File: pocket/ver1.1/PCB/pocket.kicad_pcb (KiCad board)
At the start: 2 copper layers, 225.4 x 60.3 mm, 60 parts, among them SW1 MX_SW_HS, SW10 MX_SW_HS, SW11 MX_SW_HS, SW12 MX_SW_HS, SW13 MX_SW_HS, SW14 MX_SW_HS, SW15 MX_SW_HS, SW16 MX_SW_HS, SW17 MX_SW_HS, SW18 MX_SW_HS, SW19 MX_SW_HS, SW2 MX_SW_HS, SW20 MX_SW_HS, SW21 MX_SW_HS, SW22 MX_SW_HS, SW23 MX_SW_HS, SW24 MX_SW_HS, SW25 MX_SW_HS, SW26 MX_SW_HS, SW27 MX_SW_HS, SW28 MX_SW_HS, SW29 MX_SW_HS, SW3 MX_SW_HS, SW4 MX_SW_HS, SW5 MX_SW_HS, SW6 MX_SW_HS, SW7 MX_SW_HS, SW8 MX_SW_HS, SW9 MX_SW_HS, U1 ProMicro

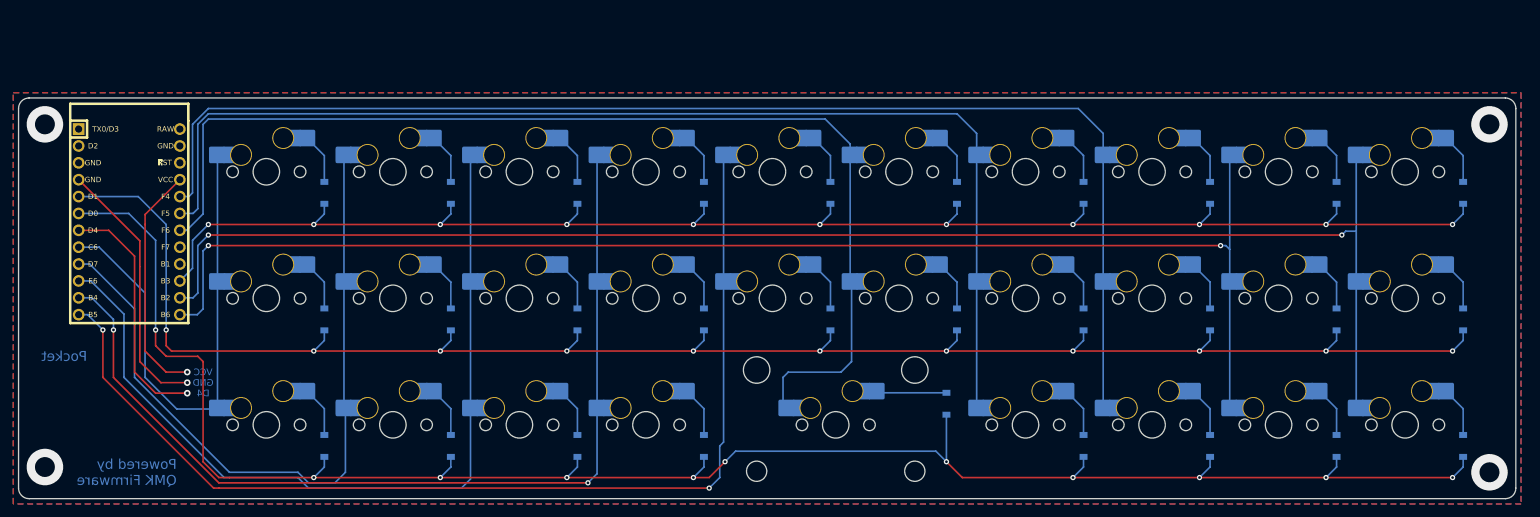
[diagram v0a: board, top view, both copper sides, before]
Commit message: Add files via upload
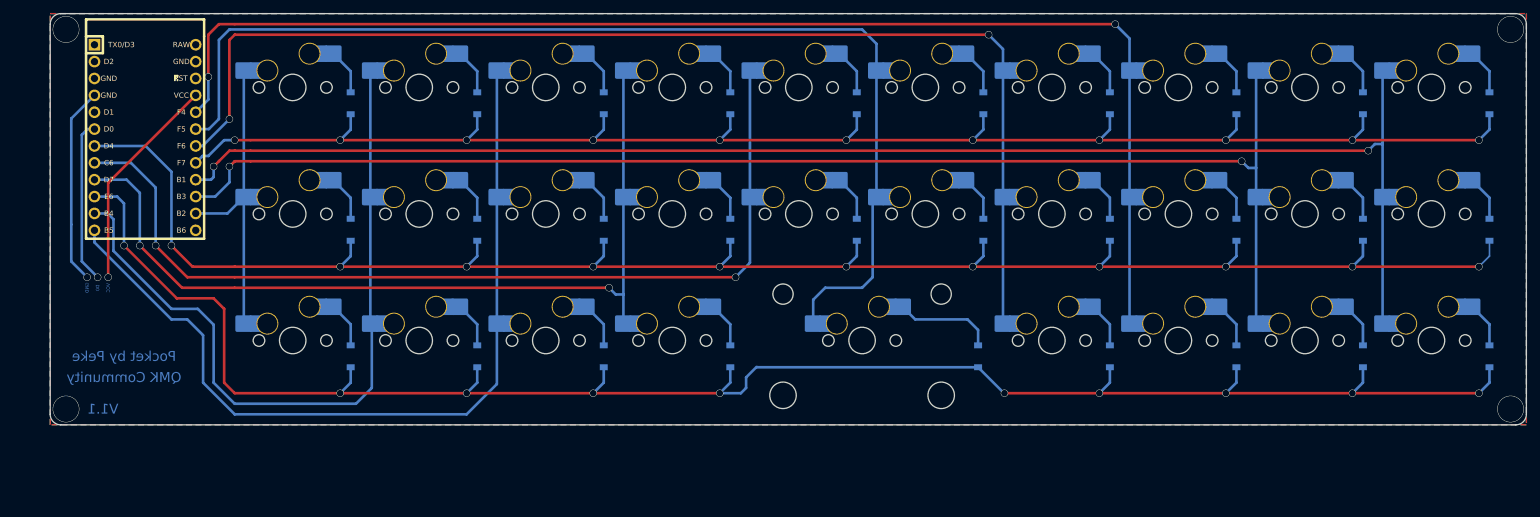
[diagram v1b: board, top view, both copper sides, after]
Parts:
- moved D1 14.1 mm to (261.1, 74.6)
- moved D10 14.1 mm to (89.7, 74.6)
- moved D11 14.1 mm to (261.1, 93.7)
- moved D12 14.1 mm to (242.1, 93.7)
- moved D13 14.1 mm to (223.0, 93.7)
- moved D14 14.1 mm to (204.0, 93.7)
- moved D15 14.1 mm to (184.9, 93.7)
- moved D16 14.1 mm to (165.9, 93.7)
- moved D17 14.1 mm to (146.8, 93.7)
- moved D18 14.1 mm to (127.8, 93.7)
- moved D19 14.1 mm to (108.7, 93.7)
- moved D2 14.1 mm to (242.1, 74.6)
- moved D20 14.1 mm to (89.7, 93.7)
- moved D3 14.1 mm to (223.0, 74.6)
- moved D4 14.1 mm to (204.0, 74.6)
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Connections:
- D1 pad 1: B3 -> F7
- D10 pad 1: B3 -> F7
- D11 pad 1: D1 -> D4
- D12 pad 1: D1 -> D4
- D13 pad 1: D1 -> D4
- D14 pad 1: D1 -> D4
- D15 pad 1: D1 -> D4
- D16 pad 1: D1 -> D4
- D17 pad 1: D1 -> D4
- D18 pad 1: D1 -> D4
- D19 pad 1: D1 -> D4
- D2 pad 1: B3 -> F7
- D20 pad 1: D1 -> D4
- D21 pad 1: D0 -> E6
- D22 pad 1: D0 -> E6
- D23 pad 1: D0 -> E6
- D24 pad 1: D0 -> E6
- D25 pad 1: D0 -> E6
- D26 pad 1: D0 -> E6
- D27 pad 1: D0 -> E6
- D28 pad 1: D0 -> E6
- D29 pad 1: D0 -> E6
- D3 pad 1: B3 -> F7
- D4 pad 1: B3 -> F7
- D5 pad 1: B3 -> F7
- D6 pad 1: B3 -> F7
- D7 pad 1: B3 -> F7
- D8 pad 1: B3 -> F7
- D9 pad 1: B3 -> F7
- SW1 pad 1: B2 -> B1
- SW10 pad 1: C6 -> B2
- SW11 pad 1: B2 -> B1
- SW12 pad 1: B6 -> B3
- SW14 pad 1: F5 -> F6
- SW15 pad 1: F6 -> F5
- SW16 pad 1: B5 -> C6
- SW17 pad 1: B4 -> D7
- SW18 pad 1: E6 -> B5
- SW19 pad 1: D7 -> B4
- SW2 pad 1: B6 -> B3
- SW20 pad 1: C6 -> B2
- SW21 pad 1: B2 -> B1
- SW22 pad 1: B6 -> B3
- SW24 pad 1: F5 -> F6
- SW25 pad 1: F6 -> F5
- SW26 pad 1: B4 -> D7
- SW27 pad 1: E6 -> B5
- SW28 pad 1: D7 -> B4
- SW29 pad 1: C6 -> B2
- SW4 pad 1: F5 -> F6
- SW5 pad 1: F6 -> F5
- SW6 pad 1: B5 -> C6
- SW7 pad 1: B4 -> D7
- SW8 pad 1: E6 -> B5
- SW9 pad 1: D7 -> B4
- U1 pad 13: B6 -> unconnected-(U1-Pad13)
- U1 pad 16: unconnected-(U1-Pad16) -> B1
- U1 pad 17: unconnected-(U1-Pad17) -> F7
- U1 pad 5: D1 -> unconnected-(U1-Pad5)
- U1 pad 6: D0 -> unconnected-(U1-Pad6)
- U1 pad 7: unconnected-(U1-Pad7) -> D4
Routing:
- net D0: track 282.0 -> 0.00 mm, vias 11 -> 0
- net D4: track 0.00 -> 268.1 mm, vias 0 -> 11
- net D1: track 264.9 -> 0.00 mm, vias 11 -> 0
- net F7: track 0.00 -> 240.3 mm, vias 0 -> 11
- net B1: track 0.00 -> 220.0 mm, vias 0 -> 2
- net B6: track 205.8 -> 0.00 mm, vias 2 -> 0
- net B2: track 223.5 -> 46.4 mm, vias 2 -> 0
- net E6: track 126.9 -> 271.7 mm, vias 0 -> 10
- net C6: track 76.6 -> 140.8 mm, vias 0 -> 2
- net unconnected-(U1-Pad7): track 36.7 -> 0.00 mm, vias 1 -> 0
- net B5: track 161.0 -> 126.4 mm, vias 2 -> 0
- net B3: track 235.3 -> 201.8 mm, vias 11 -> 2
- net B4: track 143.3 -> 110.4 mm, vias 2 -> 0
- net unconnected-(U1-Pad6): track 0.00 -> 24.7 mm, vias 0 -> 1
- net D7: track 108.4 -> 129.5 mm, vias 0 -> 2
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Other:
- board size 225.4 x 60.3 mm -> 222.2 x 61.9 mm
- board text added: "D0"
- board text added: "Pocket by Peke"
- board text added: "QMK Community"
- board text added: "V1.1"
- board text removed: "D4"
- board text removed: "Pocket"
- board text removed: "Powered by QMK Firmware"
